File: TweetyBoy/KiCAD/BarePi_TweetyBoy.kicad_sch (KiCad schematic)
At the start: 4 parts, among them IC1 CH32X035G8R6, J1 OUT, J2 WCH-LINK

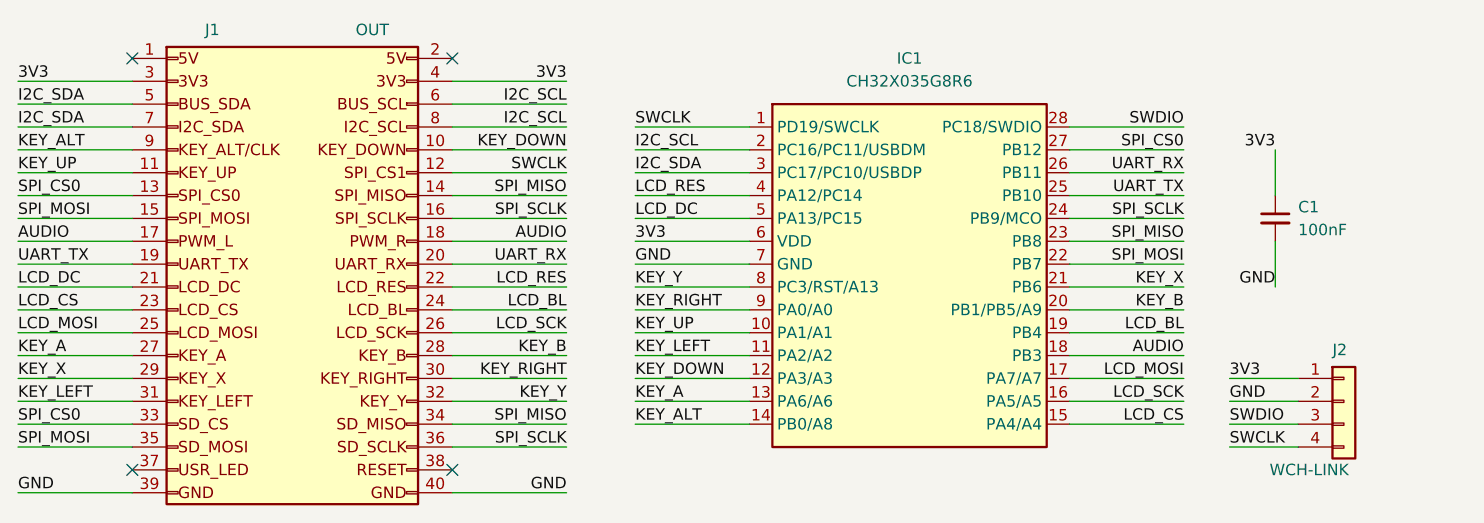
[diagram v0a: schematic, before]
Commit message: init
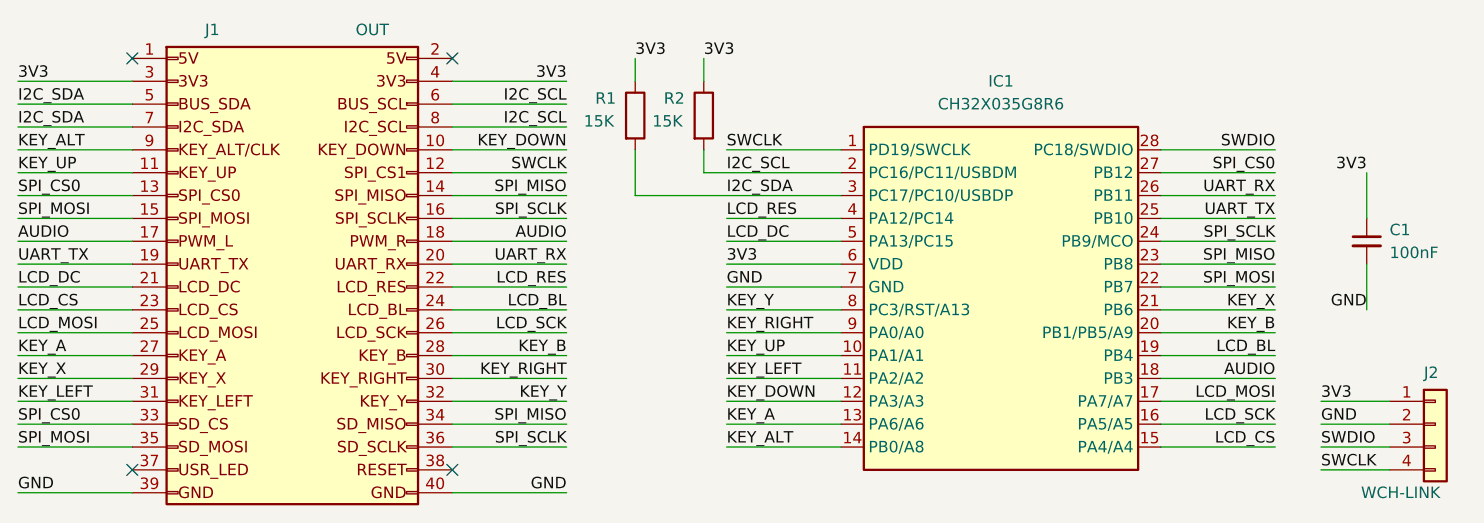
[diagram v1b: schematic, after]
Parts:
- added R1, R2: 15K, Resistor_SMD:R_1206_3216Metric_Pad1.30x1.75mm_HandSolder, symbol Device:R
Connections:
- net 3V3: now also R1.1, R2.1
- net I2C_SCL: now also R2.2
- net I2C_SDA: now also R1.2
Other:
- moved on the sheet: C1, IC1, J2
